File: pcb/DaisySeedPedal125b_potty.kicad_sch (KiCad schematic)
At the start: 5 parts, among them J6 Conn_01x20_Socket, J7 Conn_01x20_Socket

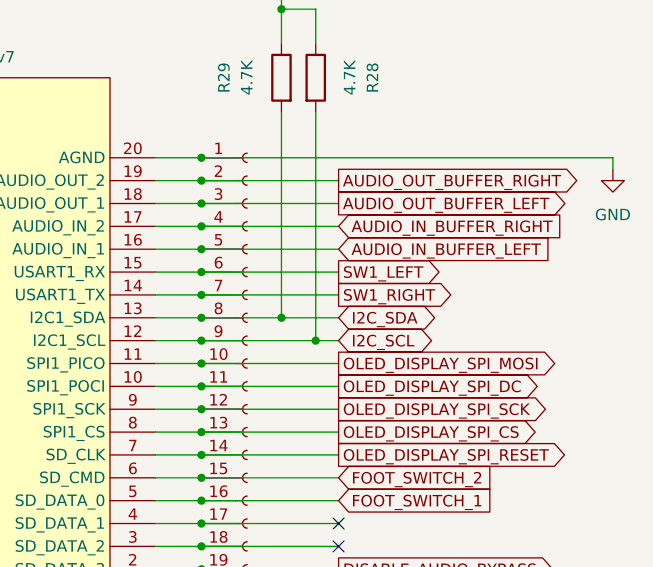
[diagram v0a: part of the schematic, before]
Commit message: Updates
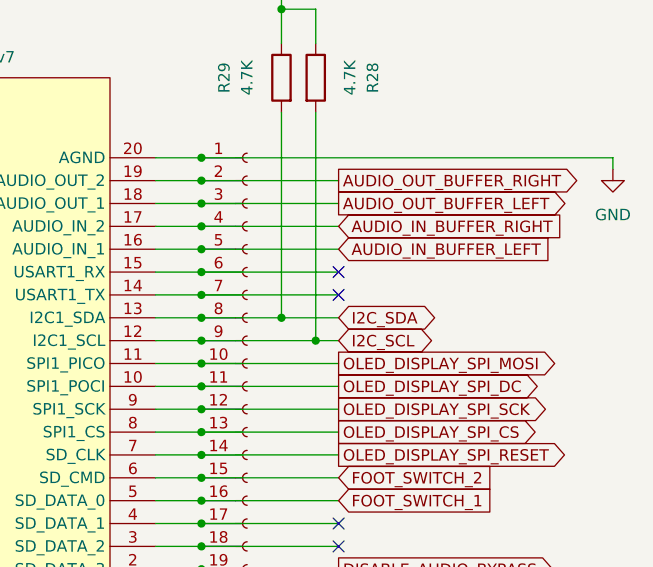
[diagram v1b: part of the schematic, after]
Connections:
- net SW1_LEFT: no longer names the net of A1.15 (USART1_RX), J7.6 (Pin_6)
- net SW1_RIGHT: no longer names the net of A1.14 (USART1_TX), J7.7 (Pin_7)
- no-connect marks 11 -> 13
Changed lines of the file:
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@@
+	)
+	(no_connect
+		(at 212.09 83.82)
 	)
 	(no_connect
@@
 	(no_connect
 		(at 212.09 116.84)
+	)
+	(no_connect
+		(at 212.09 81.28)
 	)
 	(no_connect
@@
 		)
 	)
-	(global_label "SW1_RIGHT"
-		(shape output)
-		(at 212.09 83.82 0)
-		(fields_autoplaced yes)
-		(effects
-			(font
-				(size 1.27 1.27)
-			)
-			(justify left)
-		)
-		(property "Intersheetrefs" "${INTERSHEET_REFS}"
-			(at 225.3561 83.82 0)
-			(effects
-				(font
-					(size 1.27 1.27)
-				)
-				(justify left)
-				(hide yes)
-			)
-		)
-	)
 	(global_label "OLED_DISPLAY_SPI_CS"
 		(shape output)
@@
 			(effects
 				(font
-					(size 1.27 1.27)
-				)
-				(justify left)
-				(hide yes)
-			)
-		)
-	)
-	(global_label "SW1_LEFT"
-		(shape output)
-		(at 212.09 81.28 0)
-		(fields_autoplaced yes)
-		(effects
-			(font
-				(size 1.27 1.27)
-			)
-			(justify left)
-		)
-		(property "Intersheetrefs" "${INTERSHEET_REFS}"
-			(at 224.1465 81.28 0)
-			(effects
-				(font
